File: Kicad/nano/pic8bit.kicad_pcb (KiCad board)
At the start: 2 copper layers, 21 x 52 mm, 38 parts, among them K1 MCU 1, K2 MCU 2, K3 ICSP, K4 POWER & UART, U1 PIC16F/PIC18F, U2 MCP2221A, U3 BU33SD5WG

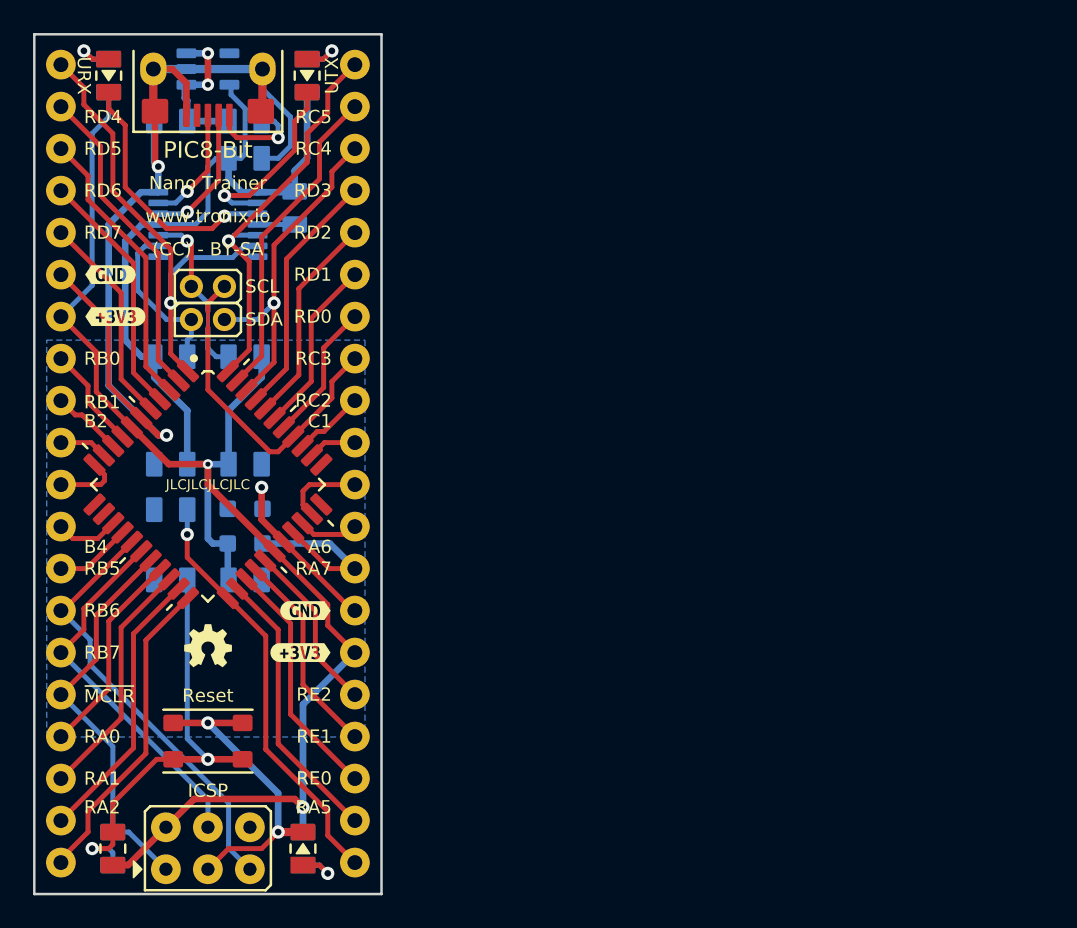
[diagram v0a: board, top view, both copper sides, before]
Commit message: Update pic8bit.kicad_pcb
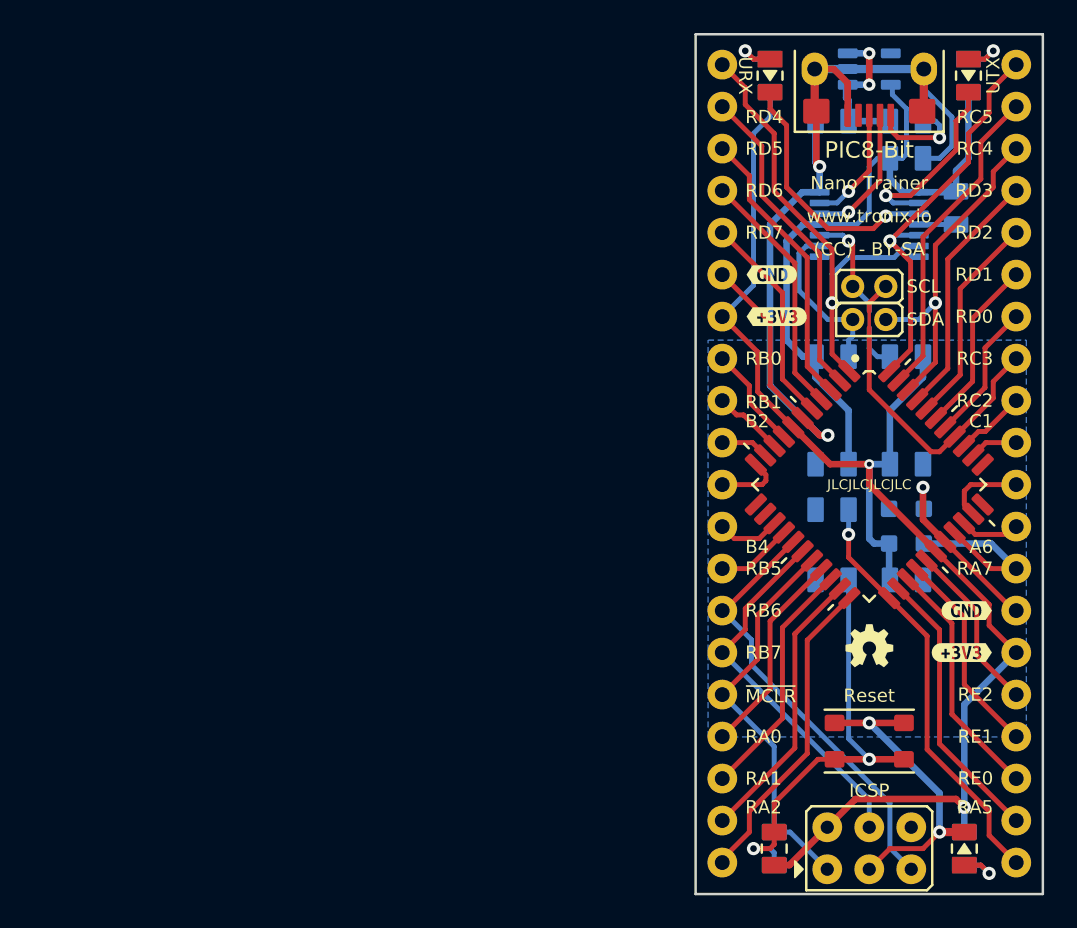
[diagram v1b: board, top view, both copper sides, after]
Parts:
- moved K1 40.0 mm to (141.6, 49.8)
- moved K3 40.0 mm to (148.0, 98.5)
- moved C1 40.0 mm to (148.2, 81.0)
- moved C2 40.0 mm to (152.8, 81.0)
- moved C3 40.0 mm to (148.2, 74.0)
- moved C4 40.0 mm to (152.8, 74.0)
- moved C5 40.0 mm to (148.2, 76.8)
- moved C7 40.0 mm to (148.2, 53.2)
- moved C8 40.0 mm to (152.8, 55.5)
- moved F1 40.0 mm to (152.8, 53.2)
- moved GB 40.0 mm to (150.5, 92.8)
- moved GT 40.0 mm to (150.5, 85.0)
- moved H1 40.0 mm to (154.0, 105.0)
- moved H2 40.0 mm to (159.1, 105.0)
- moved JP1 40.0 mm to (149.5, 63.2)
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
